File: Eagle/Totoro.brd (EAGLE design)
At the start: 105.5 x 75.2 mm, 62 parts, among them IC1 MCP6004, J1 AUDIO_JACK_3.5MMDCI, T1 BC546A

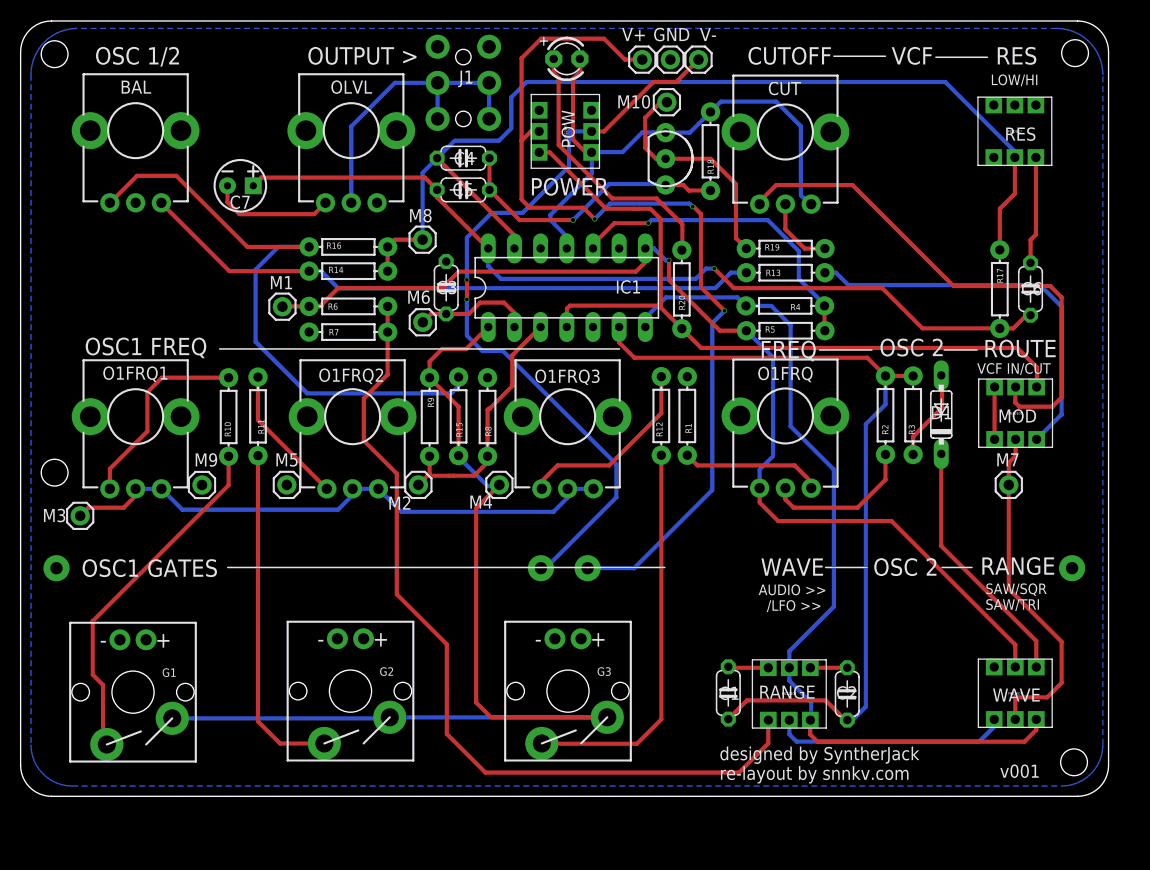
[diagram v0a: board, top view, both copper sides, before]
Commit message: hw-v010
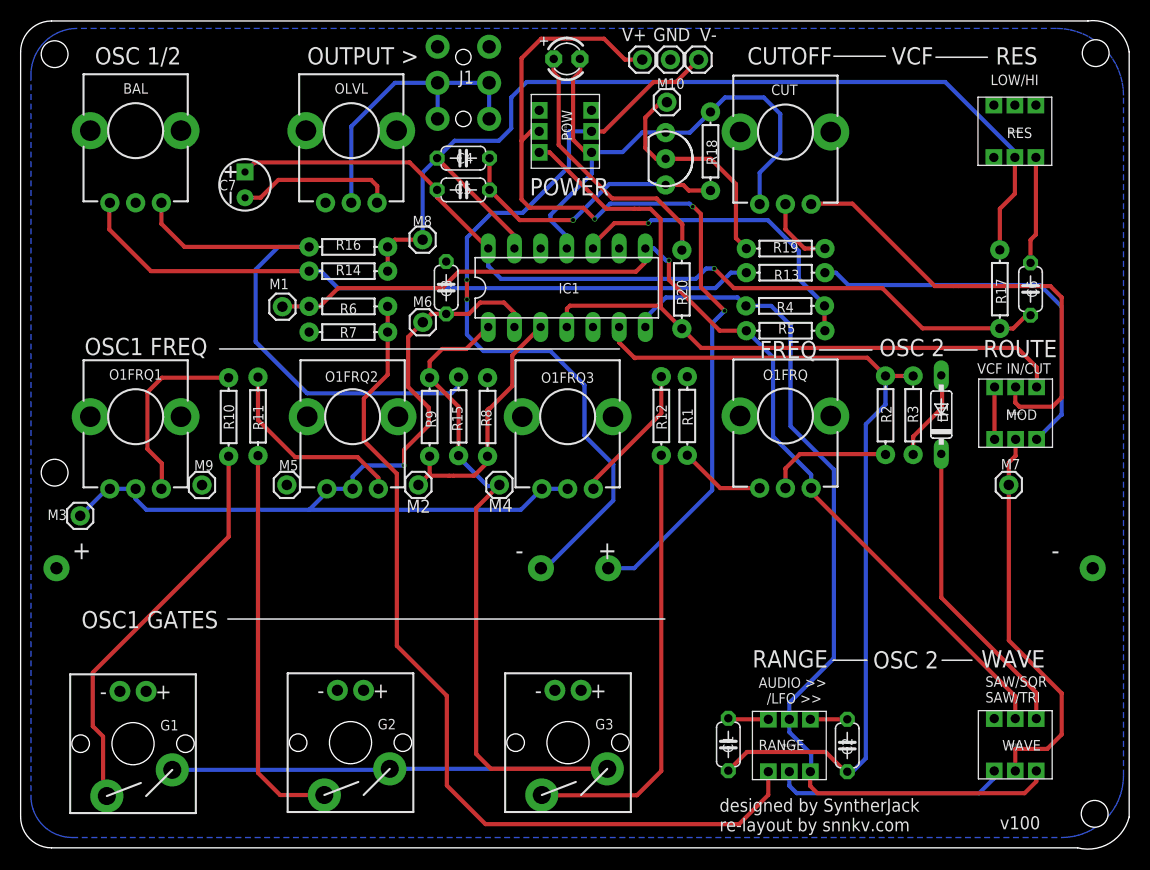
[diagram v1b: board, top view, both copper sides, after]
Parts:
- BAL, CUT, O1FRQ, O1FRQ1, O1FRQ2, O1FRQ3: value 100k(B) -> 10k
- OLVL: value 100k(A) -> 10k
- moved C2 5.00 mm to (79.2, 4.93)
- moved G2 5.00 mm to (40.5, 14.7)
- moved G3 5.00 mm to (61.6, 14.7)
- moved RANGE 5.00 mm to (71.6, 2.43)
- moved WAVE 5.00 mm to (97.5, 7.50)
- moved C1 5.00 mm to (67.7, 5.03)
- moved G1 5.00 mm to (19.4, 14.6)
- moved BATT1 2.00 mm to (78.0, 22.1)
- moved C7 0.46 mm to (20.8, 59.3), turned to 90 degrees
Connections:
- removed net N$30: M3.1, O1FRQ1.P$2, O1FRQ1.P$3, O1FRQ2.P$2, O1FRQ2.P$3, O1FRQ3.P$2, O1FRQ3.P$3
- net GND: now also OLVL.P$1; no longer OLVL.P$3
- net N$13: now also BAL.P$3; no longer BAL.P$1
- net N$14: now also BAL.P$1; no longer BAL.P$3
- net N$21: now also CUT.P$3; no longer CUT.P$1
- net N$22: now also OLVL.P$3; no longer OLVL.P$1
- net N$24: now also O1FRQ3.P$3; no longer O1FRQ3.P$1
- net N$26: now also O1FRQ2.P$3; no longer O1FRQ2.P$1
- net N$28: now also O1FRQ1.P$3; no longer O1FRQ1.P$1
- net N$3: now also O1FRQ.P$1; no longer O1FRQ.P$3
- net N$31: now also M3.1, O1FRQ1.P$1, O1FRQ1.P$2, O1FRQ2.P$1, O1FRQ2.P$2, O1FRQ3.P$1, O1FRQ3.P$2
- net N$8: now also O1FRQ.P$3; no longer O1FRQ.P$1
- net VSS: now also CUT.P$1; no longer CUT.P$3
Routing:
- net N$31: track 11.5 -> 90.4 mm, vias 0 -> 1
- net N$30: track 55.7 -> 0.00 mm
- net N$21: track 51.0 -> 44.4 mm
- net N$14: track 60.8 -> 67.4 mm
- net N$13: track 59.3 -> 53.3 mm
- net N$26: track 13.6 -> 19.2 mm
- net N$3: track 13.7 -> 8.34 mm
- net TRI_SAW: track 84.8 -> 89.8 mm
- net SQR: track 81.9 -> 86.9 mm
- net N$6: track 33.2 -> 38.2 mm
- net N$34: track 100.3 -> 105.3 mm
- net N$29: track 38.2 -> 43.2 mm
- net N$25: track 34.0 -> 39.0 mm
- net N$10: track 24.5 -> 29.5 mm
- net N$1: track 79.7 -> 84.7 mm
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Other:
- board size 105.5 x 75.2 mm -> 107.5 x 80.4 mm
- board text added: "+"
- board text added: "-"
- board text added: "v100"
- board text removed: "v001"
